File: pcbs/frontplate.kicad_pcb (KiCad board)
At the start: 2 copper layers, 133.3 x 91.7 mm, 5 parts

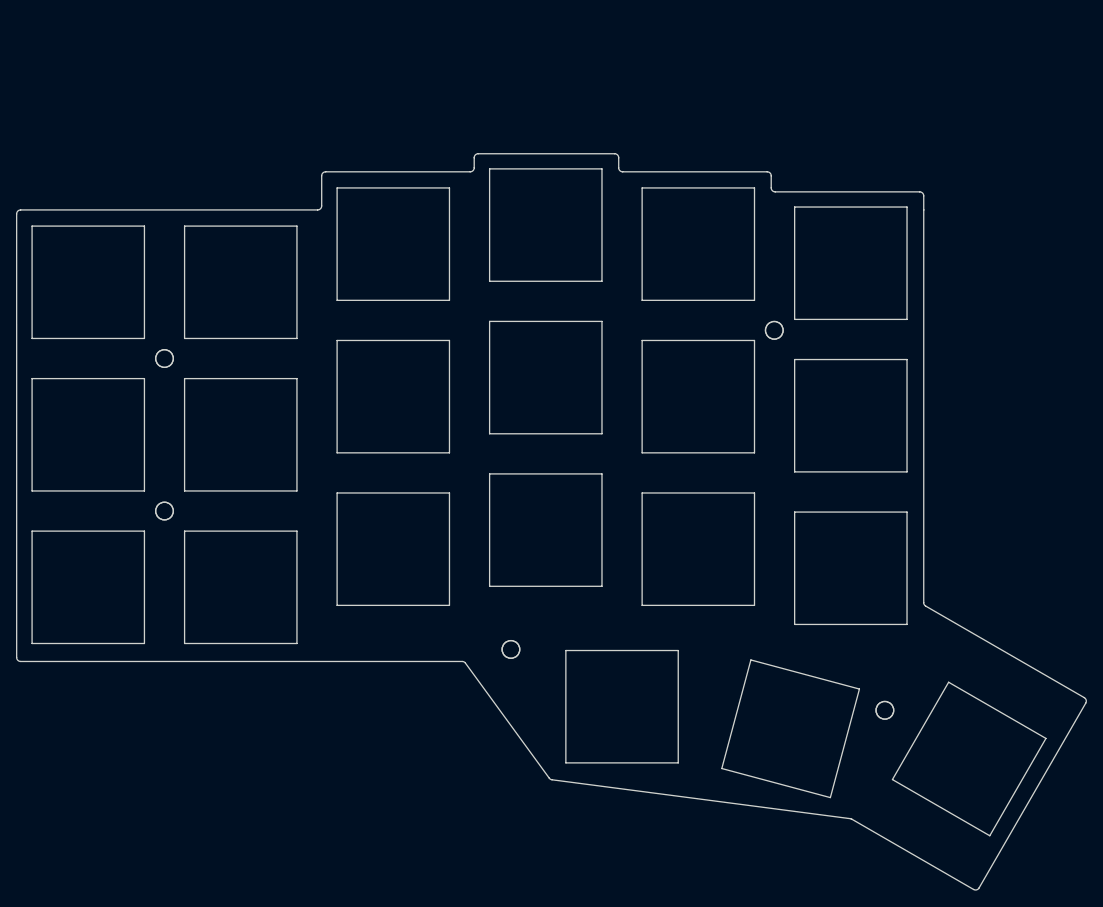
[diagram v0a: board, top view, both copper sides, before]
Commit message: feat: build script and its artifacts
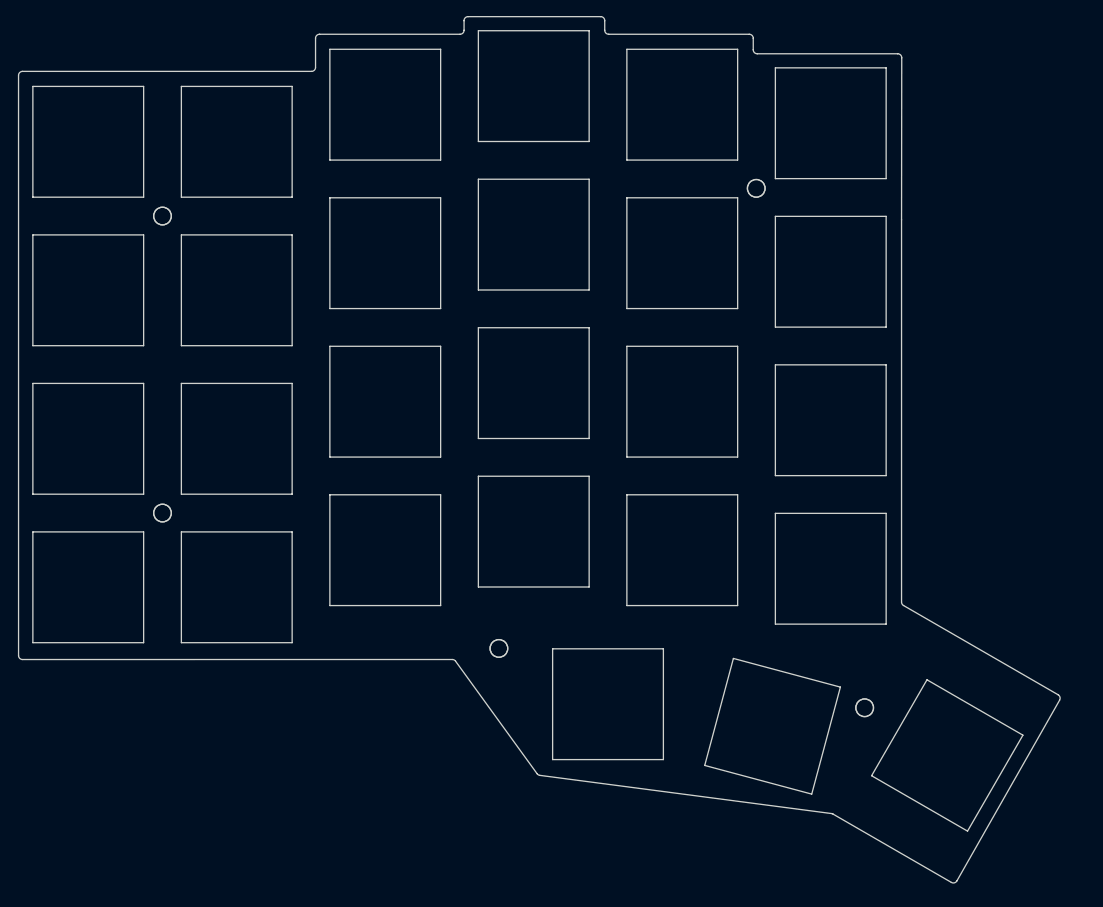
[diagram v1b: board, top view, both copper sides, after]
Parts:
- moved MH3 17.8 mm to (183.2, 50.3)
- moved MH1 17.8 mm to (109.2, 53.8)
- moved MH5 2.54 mm to (196.7, 115.0)
- moved MH4 1.51 mm to (151.2, 107.6)
- moved MH2 0.35 mm to (109.2, 90.8)
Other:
- board size 133.3 x 91.7 mm -> 129.8 x 107.9 mm
